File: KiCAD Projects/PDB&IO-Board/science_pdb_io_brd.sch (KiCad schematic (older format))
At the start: 21 parts, among them P1 ROBOT_PWR_IN, P12 ENCODER_2, P13 LIMIT1_IN, P14 LIMIT2_IN, P15 LIMIT3_IN, P16 ENCODER_3, P17 MOTOR1_PWM, P18 MOTOR2_PWM, P19 MOTOR3_PWM, P2 12V-5V_REG, P20 MOTOR4_PWM, P21 MOISTURE_CONN, P3 BBB_P9_HEADER, P4 BBB_P8_HEADER, P5 I2C_UV_Sensor, P6 I2C_Distance_Sensor, P7 SPI_Thermocouple, P8 ENCODER_1, P9 MOTOR_PWR_OUT

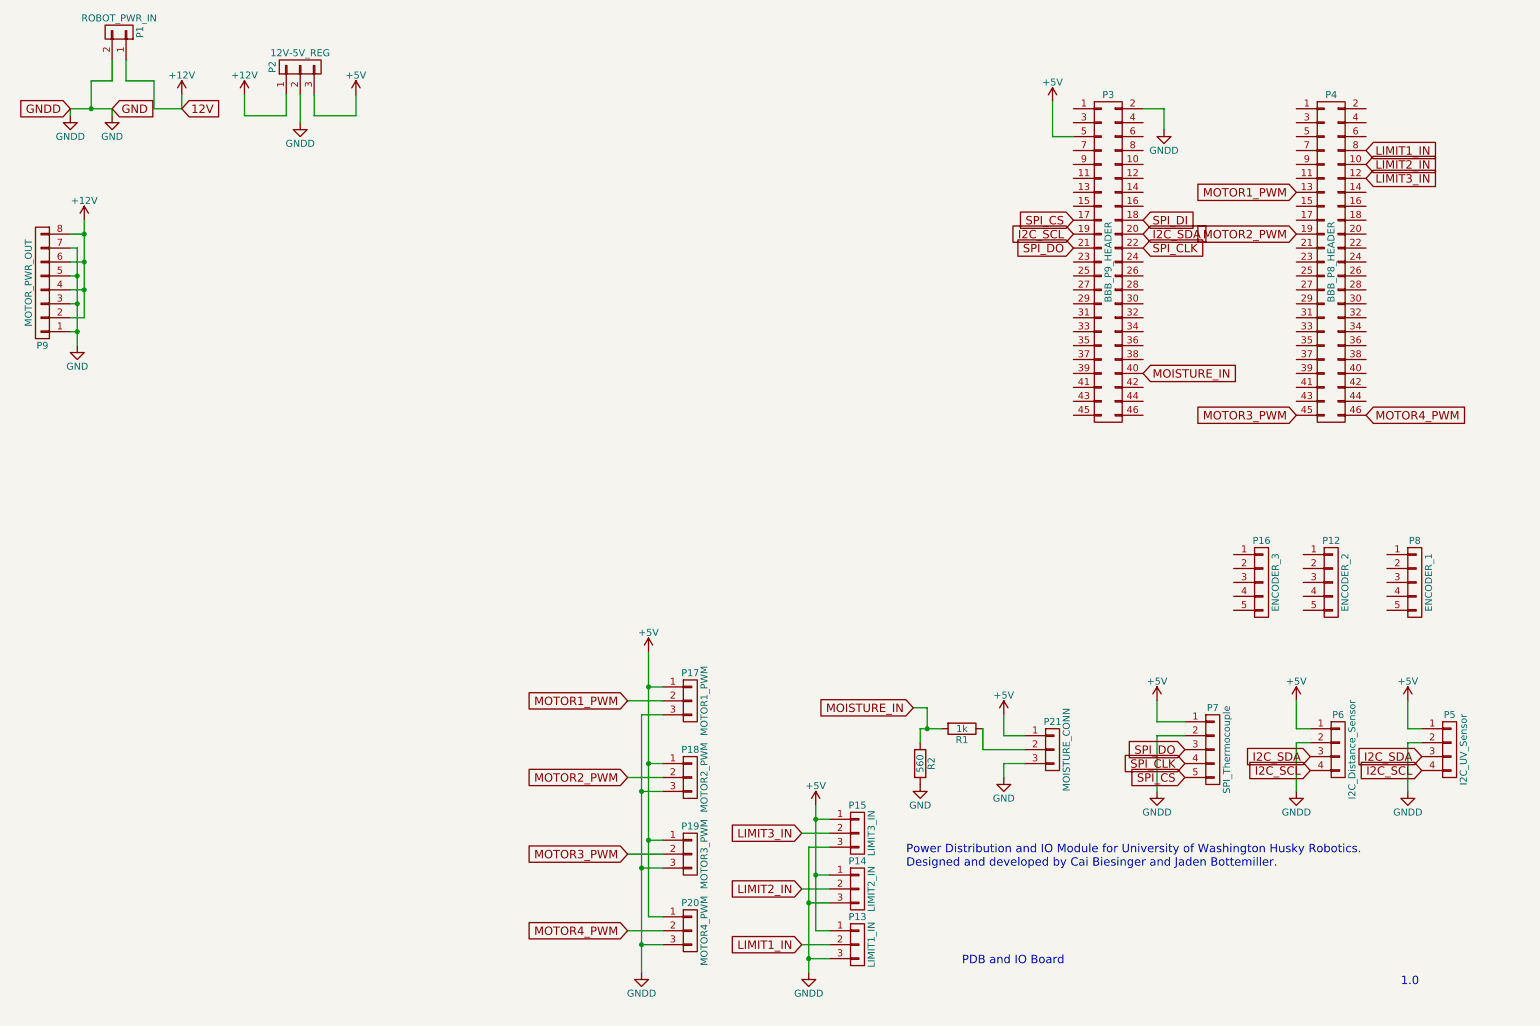
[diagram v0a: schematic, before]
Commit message: More schematic work
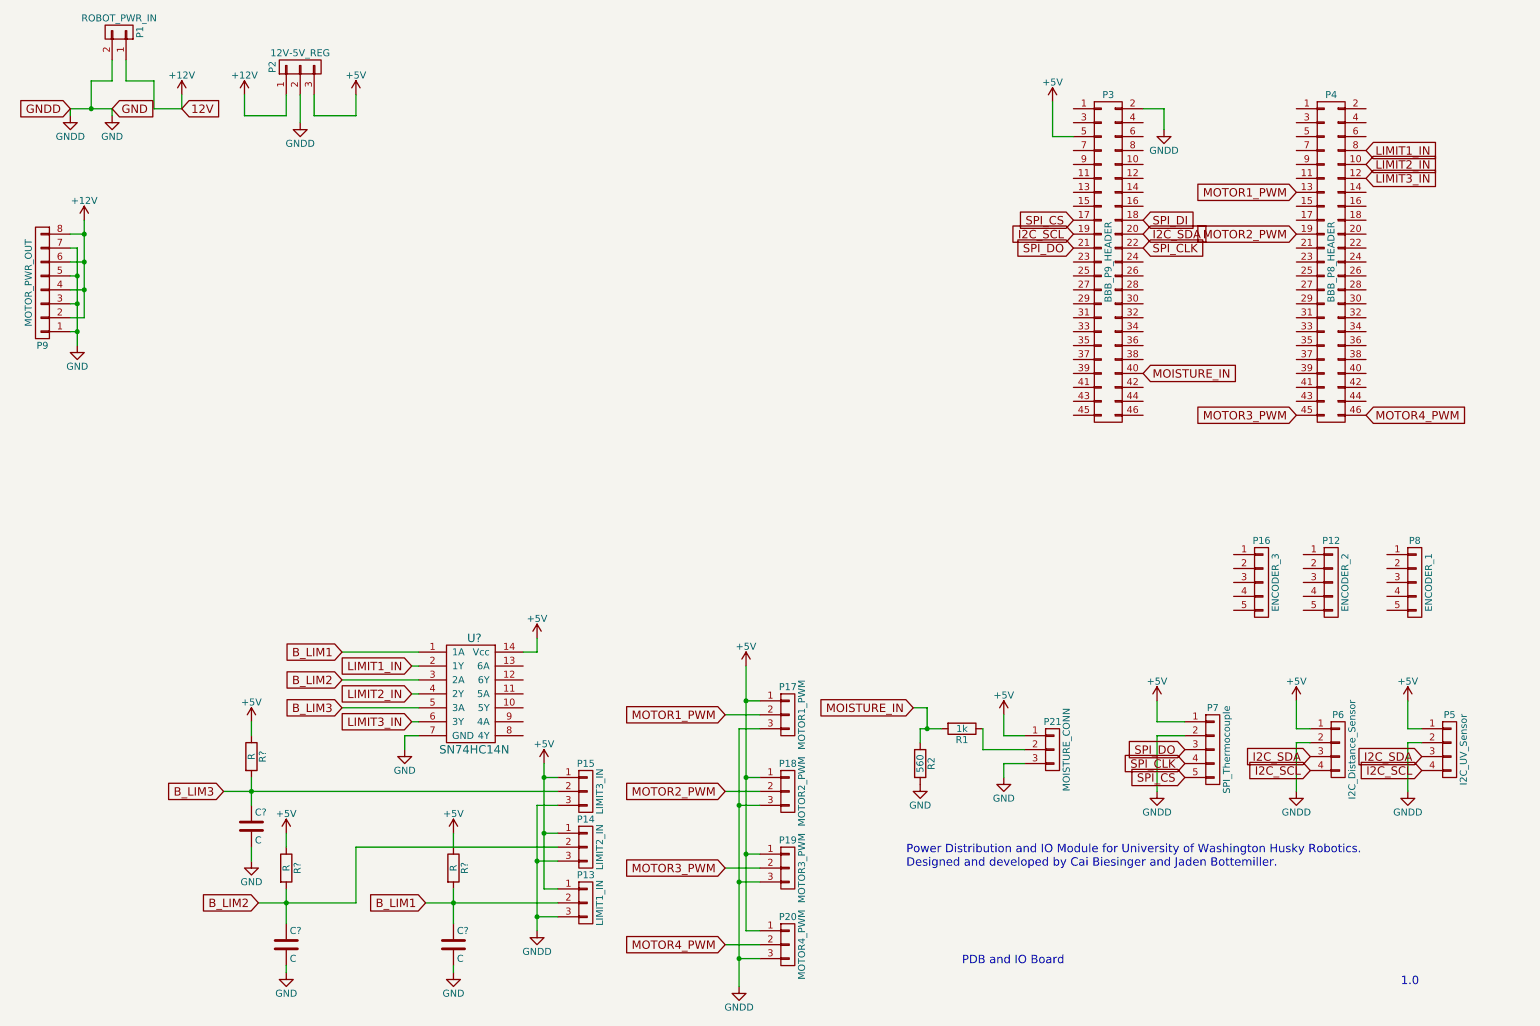
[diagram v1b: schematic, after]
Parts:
- added C? (x3): C, symbol C
- added R? (x3): R, symbol R
- added U?: SN74HC14N, symbol SN74HC14N
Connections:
- net +5V: now also R?.1, R?.1, R?.1, U?.14 (Vcc)
- net GND: now also C?.2, C?.2, C?.2, U?.7 (GND)
- net LIMIT1_IN: now also U?.2 (1Y); no longer P13.2 (P2)
- net LIMIT2_IN: now also U?.4; no longer P14.2 (P2)
- net LIMIT3_IN: now also U?.6 (3Y); no longer P15.2 (P2)
- new net B_LIM1: C?.1, P13.2 (P2), R?.2, U?.1 (1A)
- new net B_LIM2: C?.1, P14.2 (P2), R?.2, U?.3 (2A)
- new net B_LIM3: C?.1, P15.2 (P2), R?.2, U?.5 (3A)
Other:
- moved on the sheet: P13, P14, P15, P17, P18, P19, P20
